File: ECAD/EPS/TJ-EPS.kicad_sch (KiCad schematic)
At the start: 41 parts, among them J1 SWD/DEBUG, Q1 2N7002, Q2 IRF7458, U1 CD74HC4067SM, U2 CD74HC4067SM, U3 MAX6369, U4 CD74HC4067SM, U5 STM32F103C8Tx, Y1 8MHz

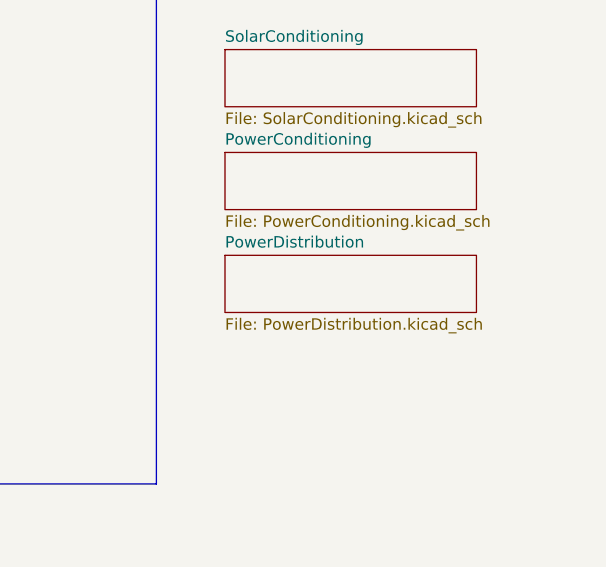
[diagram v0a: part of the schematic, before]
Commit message: selectable voltages on PDMs
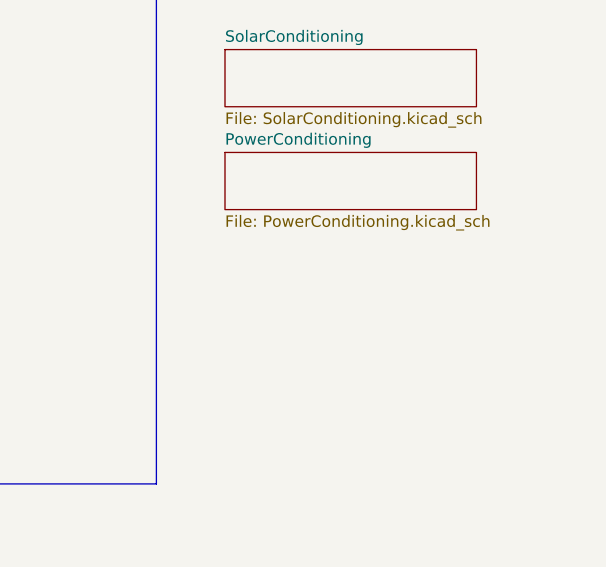
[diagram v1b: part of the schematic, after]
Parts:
- JP1: symbol TJ-EPS-rescue:SolderJumper_3_Open-Jumper -> Jumper:SolderJumper_3_Open
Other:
- removed sheet PowerDistribution

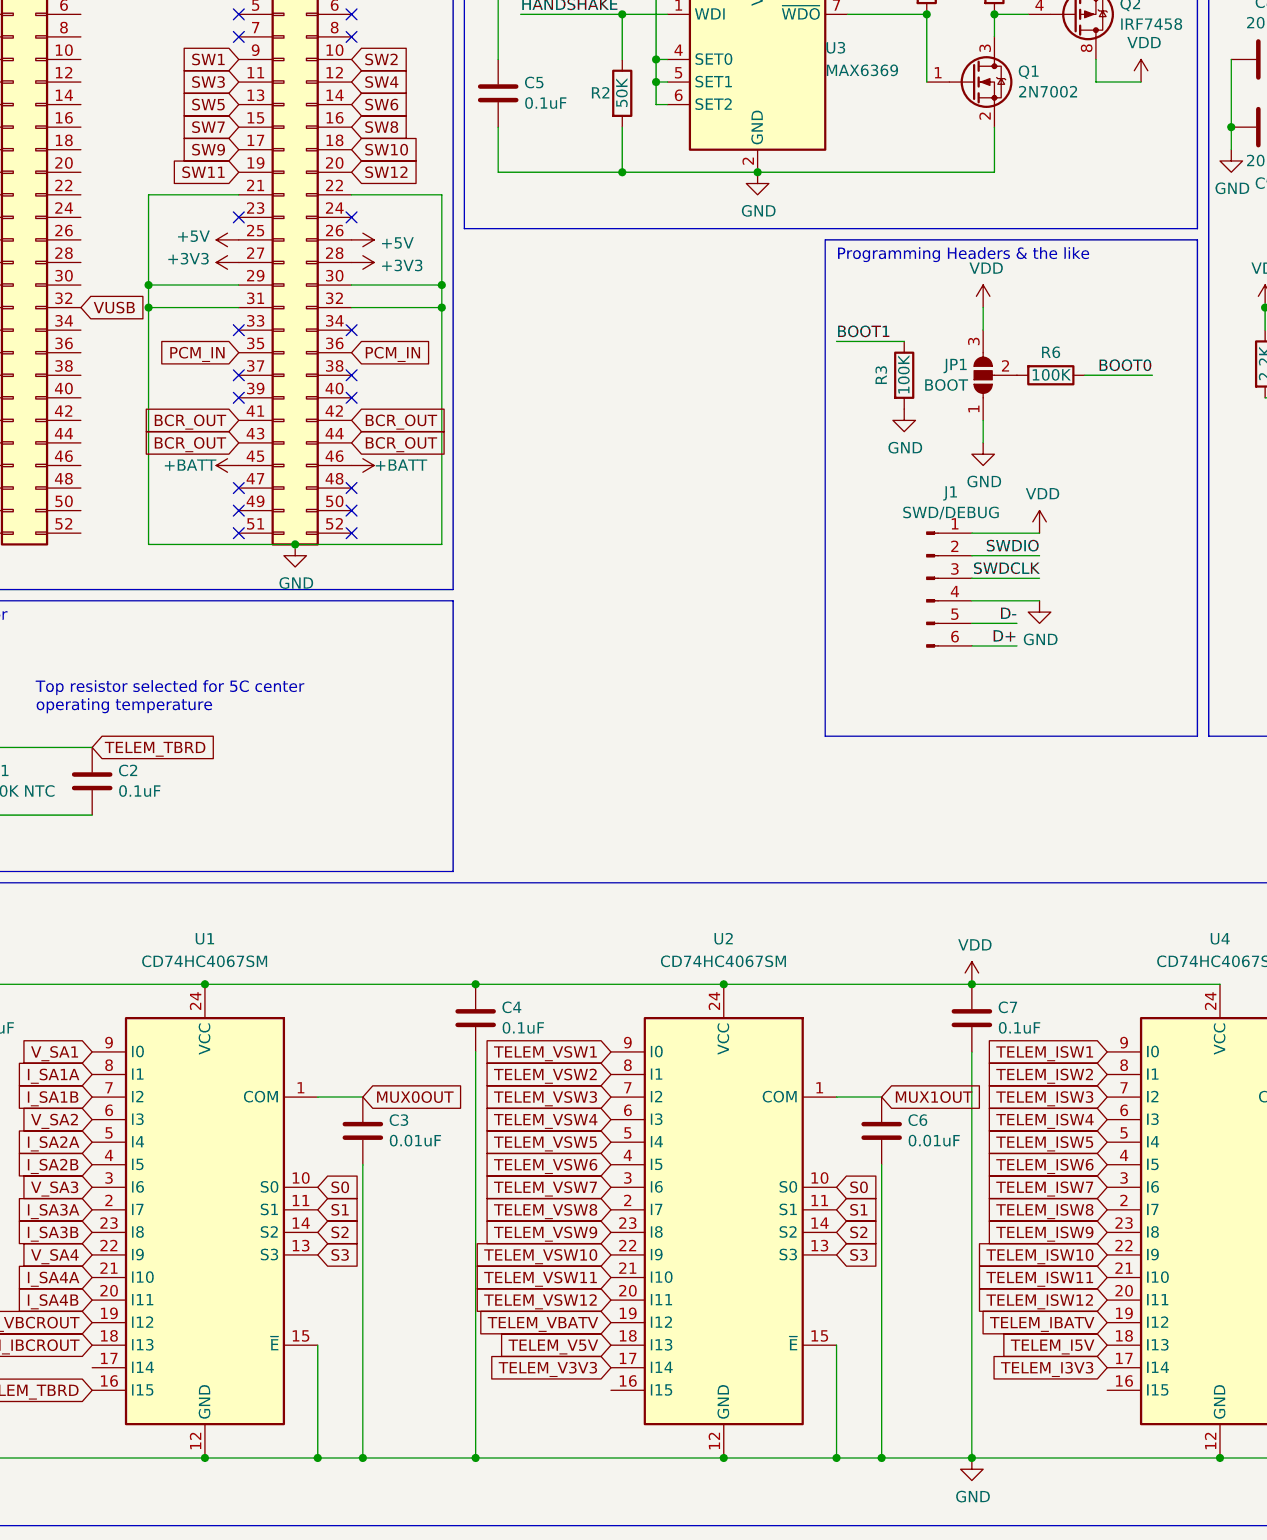
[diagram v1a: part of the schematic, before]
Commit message: descope to 10 pdms, replace mcp3208 with mcp3008 bc of stock
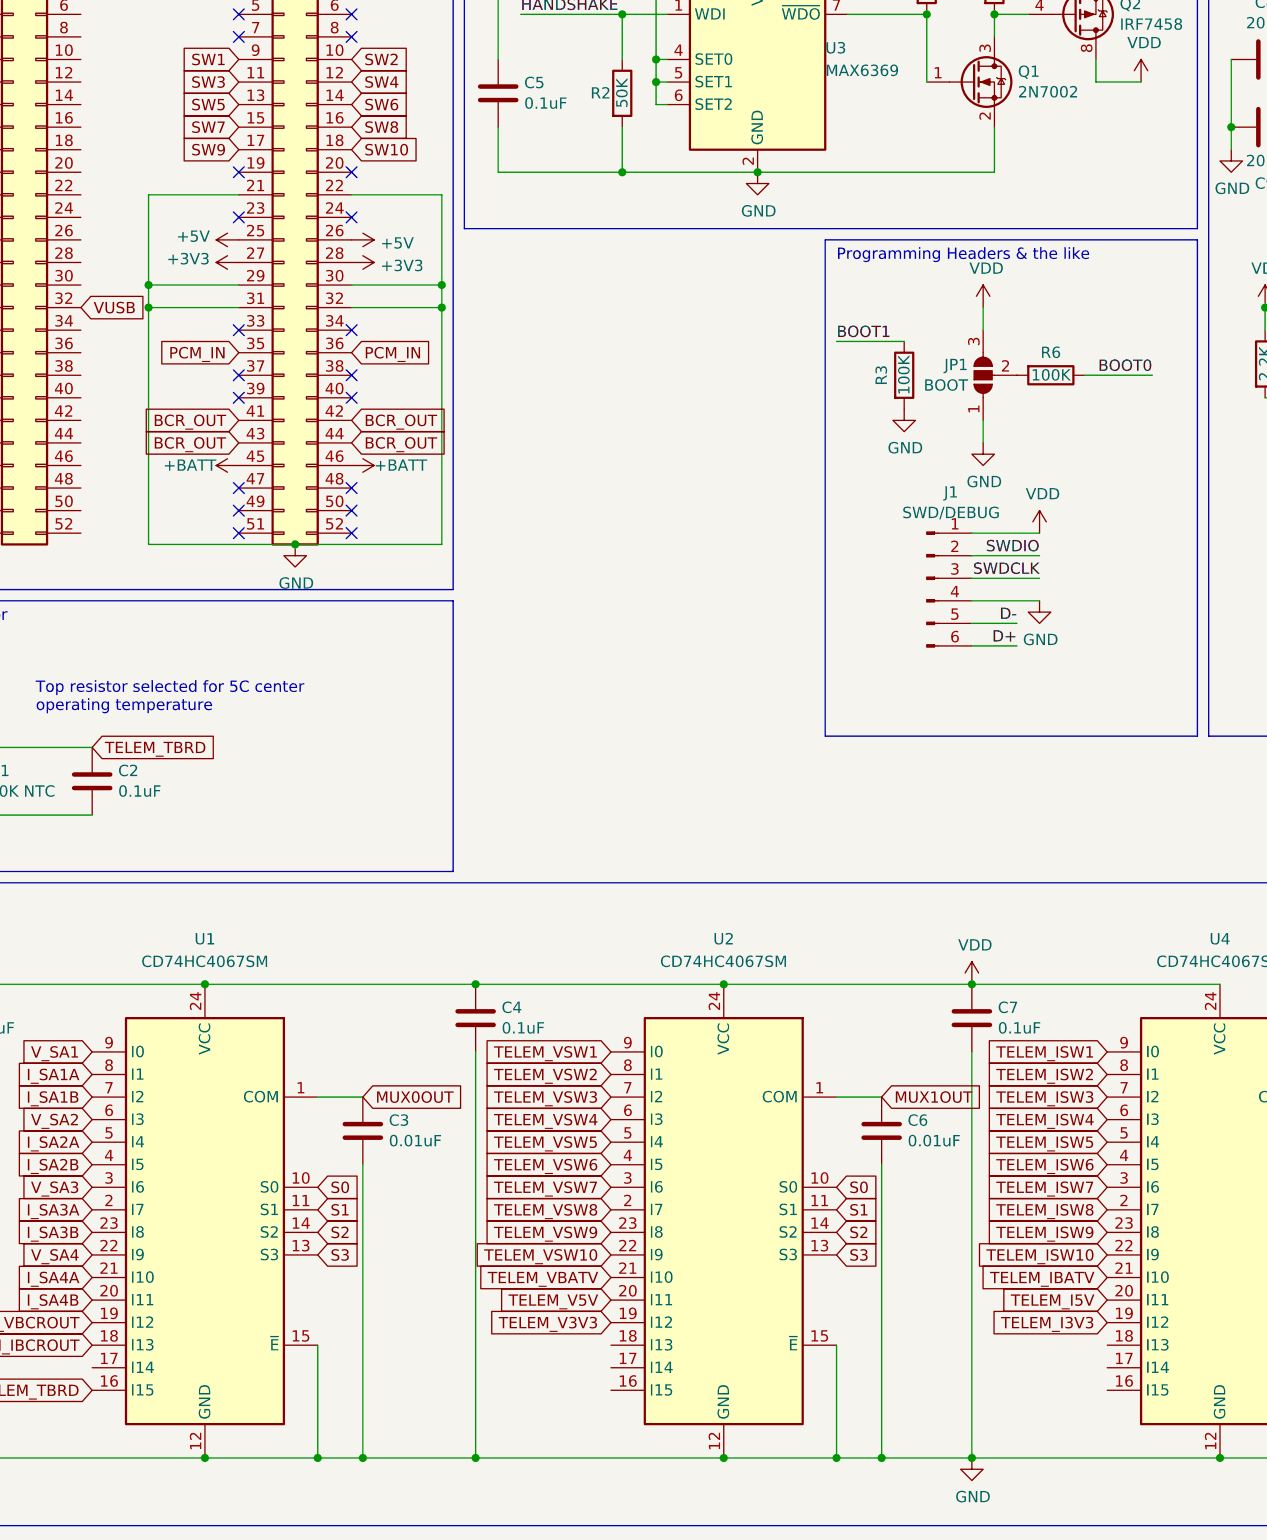
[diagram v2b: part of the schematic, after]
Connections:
- net TELEM_ISW11 is gone; now on net TELEM_IBATV: U4.21 (I10)
- net TELEM_ISW12 is gone; now on net TELEM_I5V: U4.20 (I11)
- net TELEM_VSW11 is gone; now on net TELEM_VBATV: U2.21 (I10)
- net TELEM_VSW12 is gone; now on net TELEM_V5V: U2.20 (I11)
- net TELEM_I3V3: now also U4.19 (I12); no longer U4.17 (I14)
- net TELEM_I5V: no longer U4.18 (I13)
- net TELEM_IBATV: no longer U4.19 (I12)
- net TELEM_V3V3: now also U2.19 (I12); no longer U2.17 (I14)
- net TELEM_V5V: no longer U2.18 (I13)
- net TELEM_VBATV: no longer U2.19 (I12)
- net SW11: no longer names the net of H2.19 (Pin_19)
- net SW12: no longer names the net of H2.20 (Pin_20)
- no-connect marks 22 -> 24
